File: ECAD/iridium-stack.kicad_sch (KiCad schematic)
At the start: 13 parts

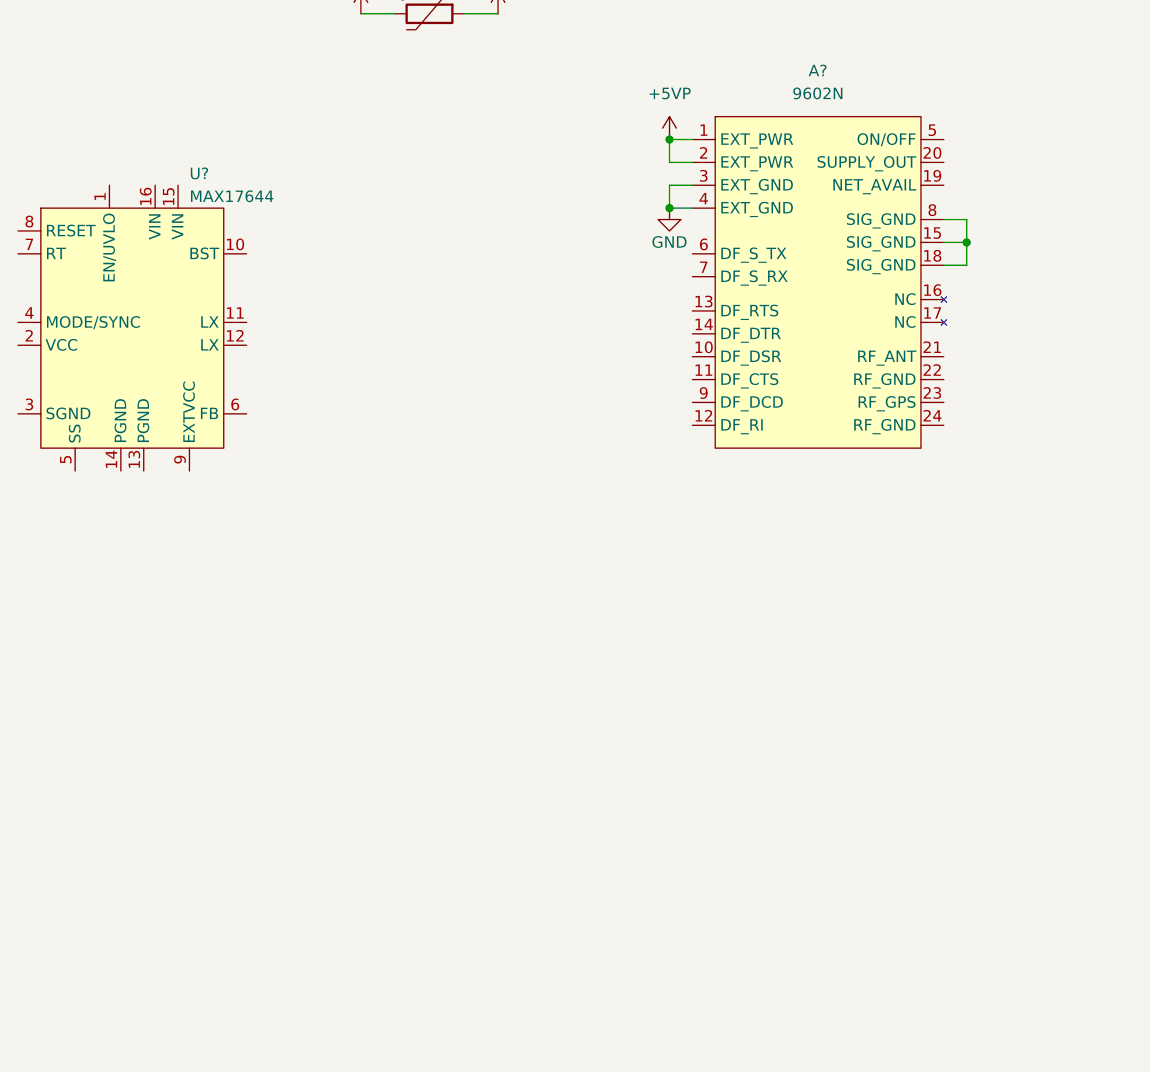
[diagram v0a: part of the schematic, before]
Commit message: Remove sync converter
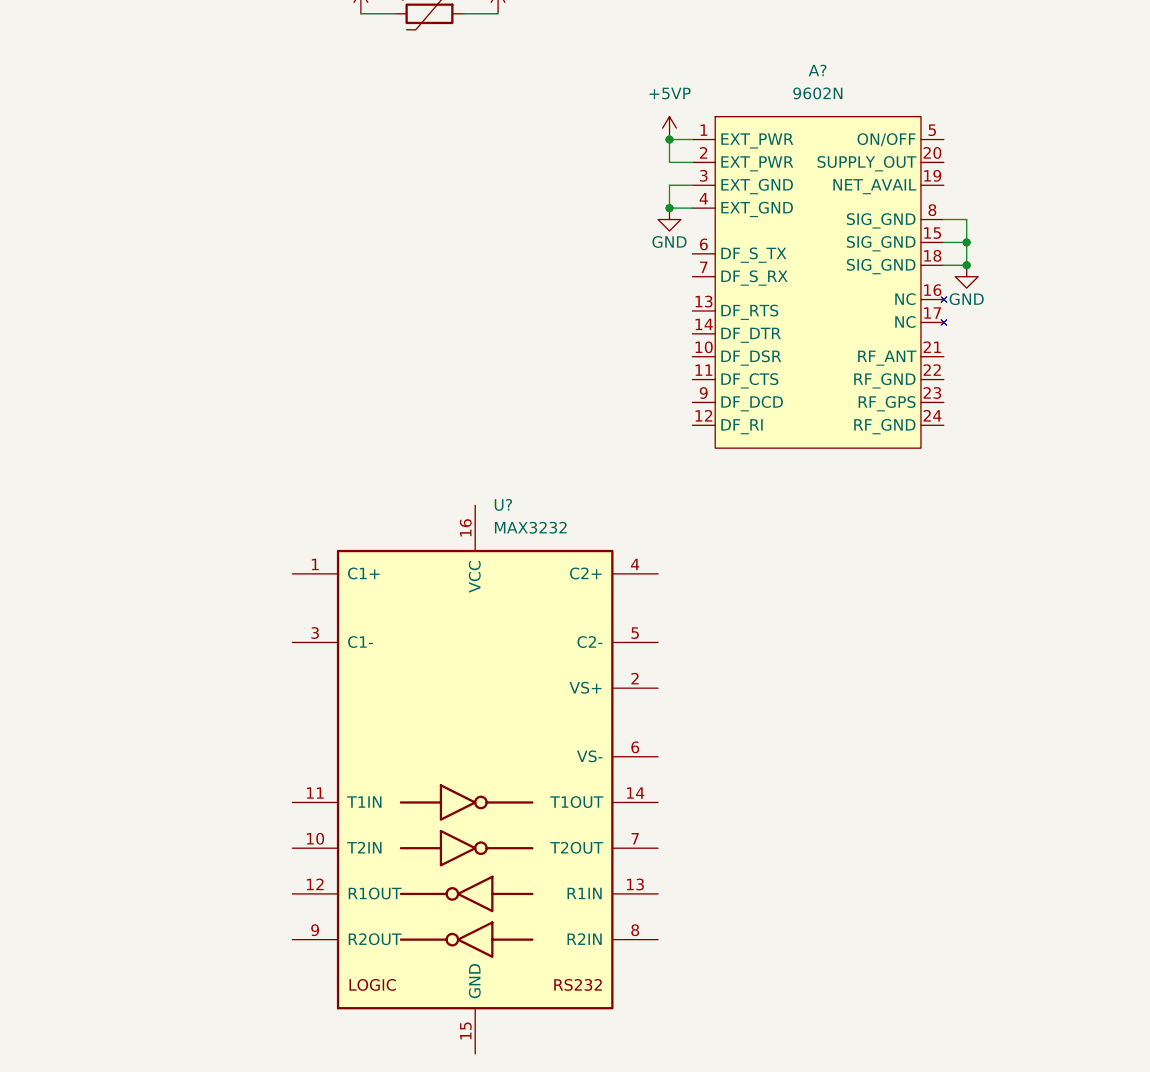
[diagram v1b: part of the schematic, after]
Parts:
- removed U?: MAX17644, symbol Symbols:MAX17644
- added U?: MAX3232, symbol Interface_UART:MAX3232
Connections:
- net GND: now also A?.15 (SIG_GND), A?.18 (SIG_GND), A?.8 (SIG_GND)
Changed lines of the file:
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@@
   (junction (at 116.84 68.58) (diameter 0) (color 0 0 0 0)
+  )
+  (junction (at 149.86 82.55) (diameter 0) (color 0 0 0 0)
   )
   (junction (at 116.84 76.2) (diameter 0) (color 0 0 0 0)
@@
     (pin "1")
   )
-  (symbol (lib_id "Symbols:MAX17644") (at 57.15 71.12 0) (unit 1)
-    (in_bom yes) (on_board yes)
-    (property "Reference" "U?" (id 0) (at 63.5 72.39 0)
-      (effects (font (size 1.27 1.27)) (justify left))
-    )
-    (property "Value" "MAX17644" (id 1) (at 63.5 74.93 0)
-      (effects (font (size 1.27 1.27)) (justify left))
-    )
-    (property "Footprint" "" (id 2) (at 57.15 71.12 0)
-      (effects (font (size 1.27 1.27)) hide)
-    )
-    (property "Datasheet" "" (id 3) (at 57.15 71.12 0)
-      (effects (font (size 1.27 1.27)) hide)
-    )
-    (pin "1")
-    (pin "10")
-    (pin "11")
-    (pin "12")
-    (pin "13")
-    (pin "14")
-    (pin "15")
-    (pin "16")
-    (pin "2")
-    (pin "3")
-    (pin "4")
-    (pin "5")
-    (pin "6")
-    (pin "7")
-    (pin "8")
-    (pin "9")
-  )
   (symbol (lib_id "power:GND") (at 116.84 76.2 0) (unit 1)
     (in_bom yes) (on_board yes)
@@
     (pin "1")
   )
+  (symbol (lib_id "power:GND") (at 149.86 82.55 0) (unit 1)
+    (in_bom yes) (on_board yes)
+    (property "Reference" "#PWR?" (id 0) (at 149.86 88.9 0)
+      (effects (font (size 1.27 1.27)) hide)
+    )
+    (property "Value" "GND" (id 1) (at 149.86 86.36 0))
+    (property "Footprint" "" (id 2) (at 149.86 82.55 0)
+      (effects (font (size 1.27 1.27)) hide)
+    )
+    (property "Datasheet" "" (id 3) (at 149.86 82.55 0)
+      (effects (font (size 1.27 1.27)) hide)
+    )
+    (pin "1")
+  )
   (symbol (lib_id "power:+5V") (at 82.55 54.61 0) (unit 1)
     (in_bom yes) (on_board yes) (fields_autoplaced)
@@
     (pin "1")
   )
+  (symbol (lib_id "Interface_UART:MAX3232") (at 95.25 139.7 0) (unit 1)
+    (in_bom yes) (on_board yes) (fields_autoplaced)
+    (property "Reference" "U?" (id 0) (at 97.2694 109.22 0)
+      (effects (font (size 1.27 1.27)) (justify left))
+    )
+    (property "Value" "MAX3232" (id 1) (at 97.2694 111.76 0)
+      (effects (font (size 1.27 1.27)) (justify left))
+    )
+    (property "Footprint" "" (id 2) (at 96.52 166.37 0)
+      (effects (font (size 1.27 1.27)) (justify left) hide)
+    )
+    (property "Datasheet" "https://datasheets.maximintegrated.com/en/ds/MAX3222-MAX3241.pdf" (id 3) (at 95.25 137.16 0)
+      (effects (font (size 1.27 1.27)) hide)
+    )
+    (pin "1")
+    (pin "10")
+    (pin "11")
+    (pin "12")
+    (pin "13")
+    (pin "14")
+    (pin "15")
+    (pin "16")
+    (pin "2")
+    (pin "3")
+    (pin "4")
+    (pin "5")
+    (pin "6")
+    (pin "7")
+    (pin "8")
+    (pin "9")
+  )
   (sheet_instances
     (path "/" (page "1"))
@@
       (reference "#PWR?") (unit 1) (value "+5VP") (footprint "")
     )
+    (path "/dc2878cb-be21-461f-b890-2b441b974fd0"
+      (reference "#PWR?") (unit 1) (value "GND") (footprint "")
+    )
     (path "/dd479a80-227b-44d6-b0fa-58cd4309c382"
       (reference "#PWR?") (unit 1) (value "+5V") (footprint "")
@@
       (reference "TH?") (unit 1) (value "NTC") (footprint "")
     )
-    (path "/02a9969f-ce81-4a97-8ae7-0a755196af14"
-      (reference "U?") (unit 1) (value "MAX17644") (footprint "")
-    )
-  )
+    (path "/fe2c9782-2ff0-473c-98b0-ea9a985143fb"
+      (reference "U?") (unit 1) (value "MAX3232") (footprint "")
+    )
+  )

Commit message: Revert "Remove sync converter"
This reverts commit 1ebd4765432d8d92d6eda4bb4eca3aef03c5145b.
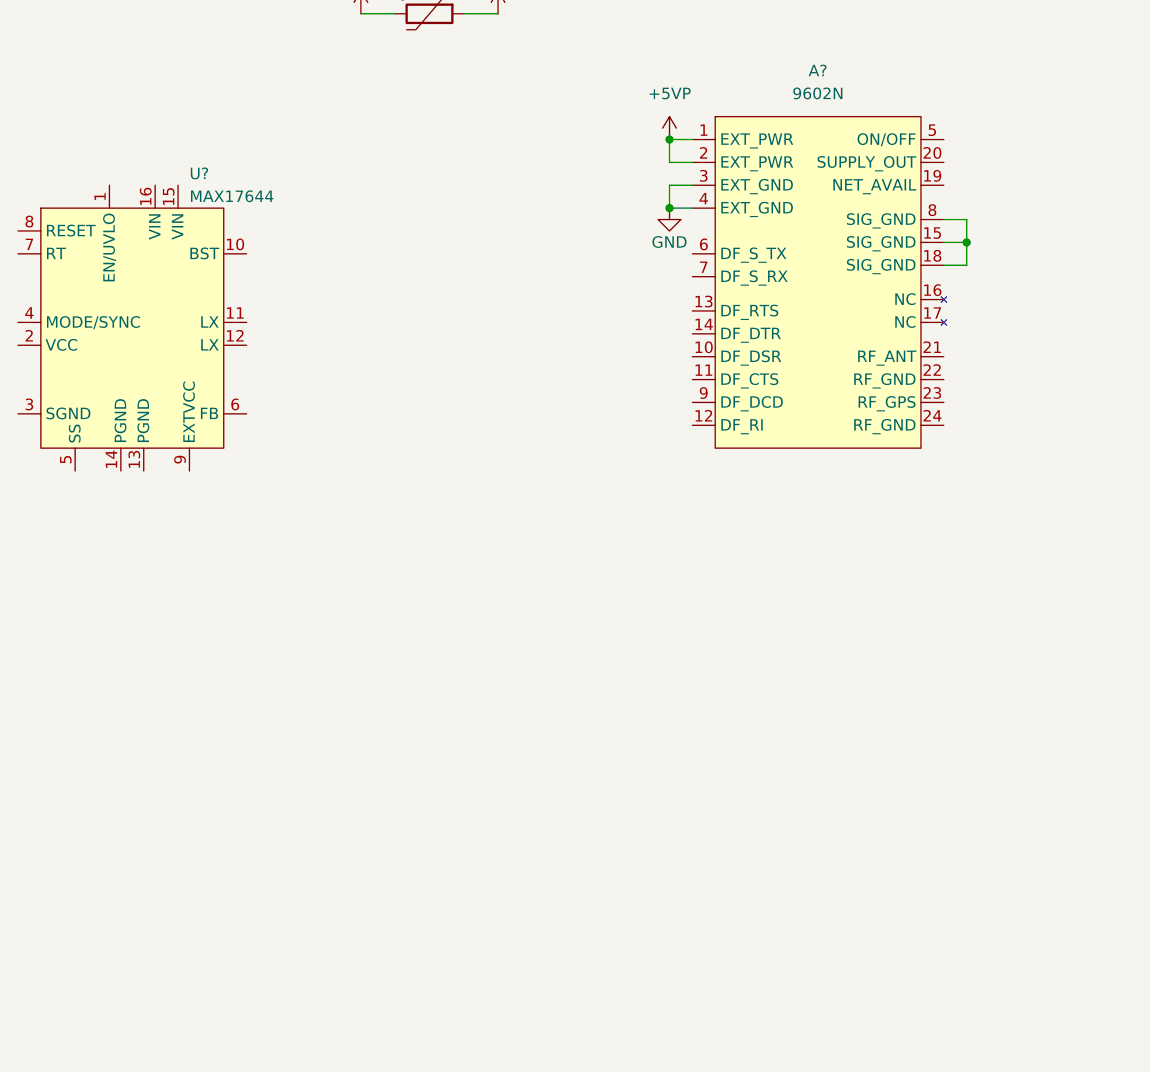
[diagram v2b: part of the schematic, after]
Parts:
- removed U?: MAX3232, symbol Interface_UART:MAX3232
- added U?: MAX17644, symbol Symbols:MAX17644
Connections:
- net GND: no longer A?.15 (SIG_GND), A?.18 (SIG_GND), A?.8 (SIG_GND)
- new net: A?.15 (SIG_GND), A?.18 (SIG_GND), A?.8 (SIG_GND)
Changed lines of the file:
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@@
   (junction (at 116.84 68.58) (diameter 0) (color 0 0 0 0)
-  )
-  (junction (at 149.86 82.55) (diameter 0) (color 0 0 0 0)
   )
   (junction (at 116.84 76.2) (diameter 0) (color 0 0 0 0)
@@
     (pin "1")
   )
+  (symbol (lib_id "Symbols:MAX17644") (at 57.15 71.12 0) (unit 1)
+    (in_bom yes) (on_board yes)
+    (property "Reference" "U?" (id 0) (at 63.5 72.39 0)
+      (effects (font (size 1.27 1.27)) (justify left))
+    )
+    (property "Value" "MAX17644" (id 1) (at 63.5 74.93 0)
+      (effects (font (size 1.27 1.27)) (justify left))
+    )
+    (property "Footprint" "" (id 2) (at 57.15 71.12 0)
+      (effects (font (size 1.27 1.27)) hide)
+    )
+    (property "Datasheet" "" (id 3) (at 57.15 71.12 0)
+      (effects (font (size 1.27 1.27)) hide)
+    )
+    (pin "1")
+    (pin "10")
+    (pin "11")
+    (pin "12")
+    (pin "13")
+    (pin "14")
+    (pin "15")
+    (pin "16")
+    (pin "2")
+    (pin "3")
+    (pin "4")
+    (pin "5")
+    (pin "6")
+    (pin "7")
+    (pin "8")
+    (pin "9")
+  )
   (symbol (lib_id "power:GND") (at 116.84 76.2 0) (unit 1)
     (in_bom yes) (on_board yes)
@@
     (pin "1")
   )
-  (symbol (lib_id "power:GND") (at 149.86 82.55 0) (unit 1)
-    (in_bom yes) (on_board yes)
-    (property "Reference" "#PWR?" (id 0) (at 149.86 88.9 0)
-      (effects (font (size 1.27 1.27)) hide)
-    )
-    (property "Value" "GND" (id 1) (at 149.86 86.36 0))
-    (property "Footprint" "" (id 2) (at 149.86 82.55 0)
-      (effects (font (size 1.27 1.27)) hide)
-    )
-    (property "Datasheet" "" (id 3) (at 149.86 82.55 0)
-      (effects (font (size 1.27 1.27)) hide)
-    )
-    (pin "1")
-  )
   (symbol (lib_id "power:+5V") (at 82.55 54.61 0) (unit 1)
     (in_bom yes) (on_board yes) (fields_autoplaced)
@@
     (pin "1")
   )
-  (symbol (lib_id "Interface_UART:MAX3232") (at 95.25 139.7 0) (unit 1)
-    (in_bom yes) (on_board yes) (fields_autoplaced)
-    (property "Reference" "U?" (id 0) (at 97.2694 109.22 0)
-      (effects (font (size 1.27 1.27)) (justify left))
-    )
-    (property "Value" "MAX3232" (id 1) (at 97.2694 111.76 0)
-      (effects (font (size 1.27 1.27)) (justify left))
-    )
-    (property "Footprint" "" (id 2) (at 96.52 166.37 0)
-      (effects (font (size 1.27 1.27)) (justify left) hide)
-    )
-    (property "Datasheet" "https://datasheets.maximintegrated.com/en/ds/MAX3222-MAX3241.pdf" (id 3) (at 95.25 137.16 0)
-      (effects (font (size 1.27 1.27)) hide)
-    )
-    (pin "1")
-    (pin "10")
-    (pin "11")
-    (pin "12")
-    (pin "13")
-    (pin "14")
-    (pin "15")
-    (pin "16")
-    (pin "2")
-    (pin "3")
-    (pin "4")
-    (pin "5")
-    (pin "6")
-    (pin "7")
-    (pin "8")
-    (pin "9")
-  )
   (sheet_instances
     (path "/" (page "1"))
@@
       (reference "#PWR?") (unit 1) (value "+5VP") (footprint "")
     )
-    (path "/dc2878cb-be21-461f-b890-2b441b974fd0"
-      (reference "#PWR?") (unit 1) (value "GND") (footprint "")
-    )
     (path "/dd479a80-227b-44d6-b0fa-58cd4309c382"
       (reference "#PWR?") (unit 1) (value "+5V") (footprint "")
@@
       (reference "TH?") (unit 1) (value "NTC") (footprint "")
     )
-    (path "/fe2c9782-2ff0-473c-98b0-ea9a985143fb"
-      (reference "U?") (unit 1) (value "MAX3232") (footprint "")
-    )
-  )
+    (path "/02a9969f-ce81-4a97-8ae7-0a755196af14"
+      (reference "U?") (unit 1) (value "MAX17644") (footprint "")
+    )
+  )
